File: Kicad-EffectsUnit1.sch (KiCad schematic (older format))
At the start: 109 parts, among them J101 In7, J102 Doepfer connector, J103 Vin 7-12v, J104 In6, J105 In3, J106 Out10, J107 Out11, J108 Out12, J109 Out13, J110 Power Conn, SW101 Dist 10, SW102 Crush A3, SW103 Rotary_Encoder_Switch, SW104 Dist 12, U101 TL072, U102 TL072

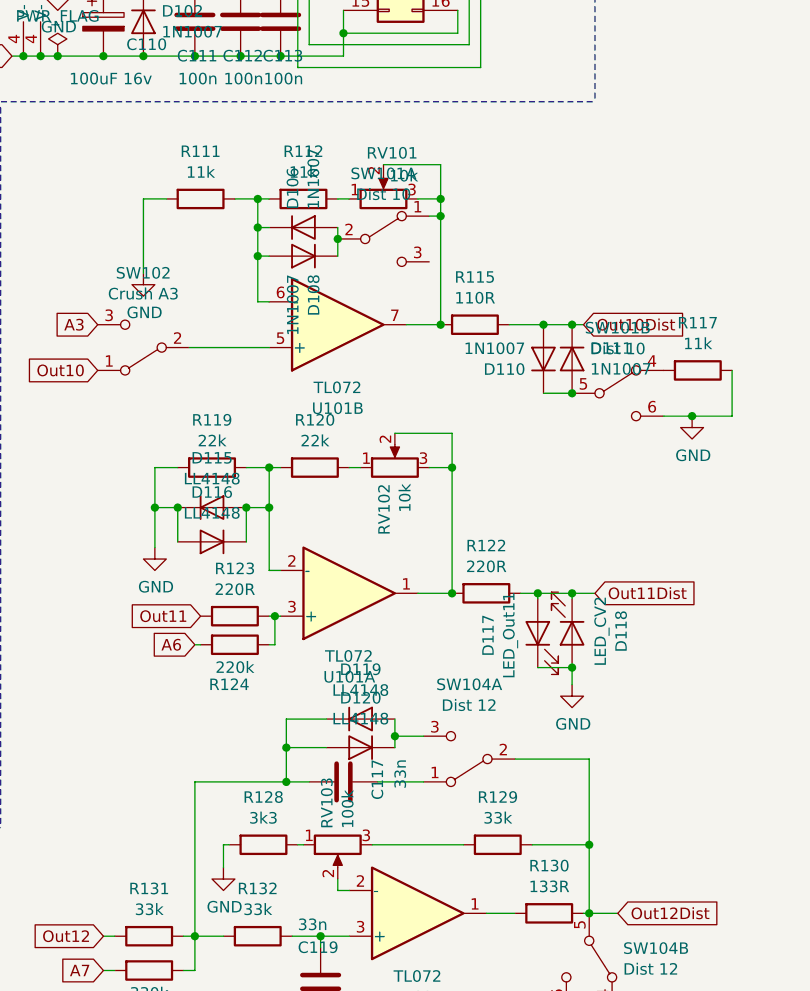
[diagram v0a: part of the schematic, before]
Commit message: Footprints
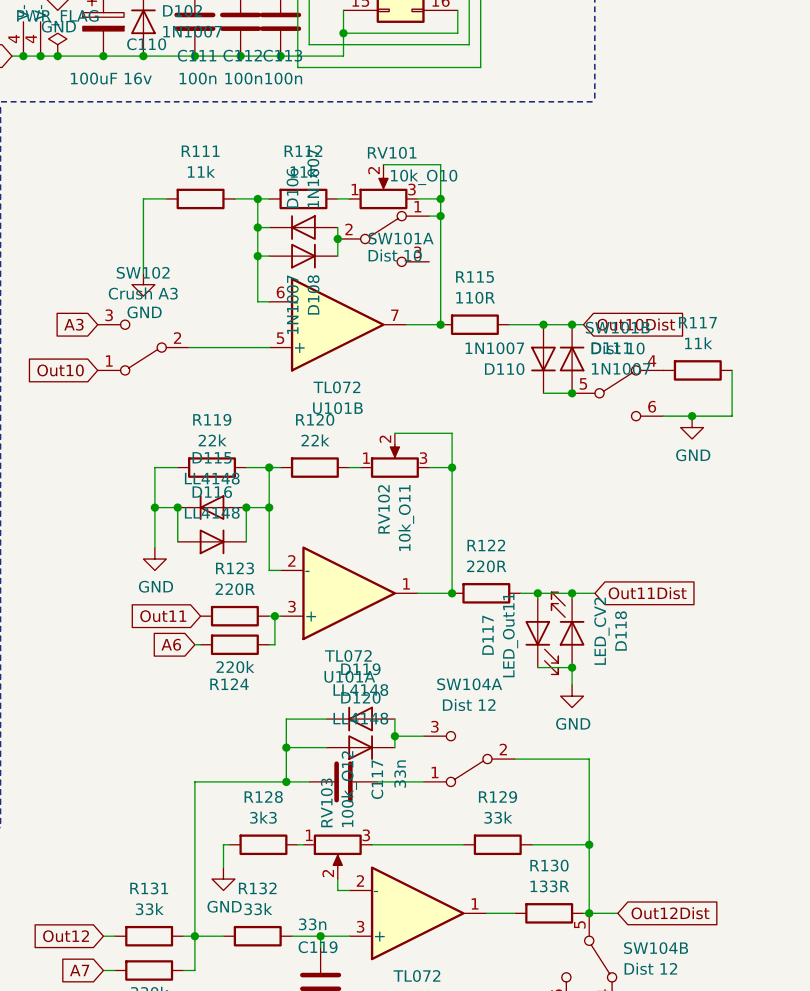
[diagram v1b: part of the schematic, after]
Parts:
- RV101: value 10k -> 10k_O10; footprint Potentiometer_THT:Potentiometer_Alps_RK09K_Single_Vertical -> Potentiometer_THT:Potentiometer_China_RK09_Single_Vertical_AJ
- RV102: value 10k -> 10k_O11; footprint Potentiometer_THT:Potentiometer_Alps_RK09K_Single_Vertical -> Potentiometer_THT:Potentiometer_China_RK09_Single_Vertical_AJ
- RV103: value 100k -> 100k_O12; footprint Potentiometer_THT:Potentiometer_Alps_RK09K_Single_Vertical -> Potentiometer_THT:Potentiometer_China_RK09_Single_Vertical_AJ
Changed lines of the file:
@@
 P 5375 3400
 F 0 "RV102" H 5305 3446 50  0000 R CNN
-F 1 "10k" H 5305 3355 50  0000 R CNN
-F 2 "Potentiometer_THT:Potentiometer_Alps_RK09K_Single_Vertical" H 5375 3400 50  0001 C CNN
+F 1 "10k_O11" H 5305 3355 50  0000 R CNN
+F 2 "Potentiometer_THT:Potentiometer_China_RK09_Single_Vertical_AJ" H 5375 3400 50  0001 C CNN
 F 3 "~" H 5375 3400 50  0001 C CNN
 	1    5375 3400
@@
 P 5325 2225
 F 0 "RV101" V 5525 2300 50  0000 R CNN
-F 1 "10k" V 5425 2200 50  0000 R CNN
-F 2 "Potentiometer_THT:Potentiometer_Alps_RK09K_Single_Vertical" H 5325 2225 50  0001 C CNN
+F 1 "10k_O10" V 5425 2200 50  0000 R CNN
+F 2 "Potentiometer_THT:Potentiometer_China_RK09_Single_Vertical_AJ" H 5325 2225 50  0001 C CNN
 F 3 "~" H 5325 2225 50  0001 C CNN
 	1    5325 2225
@@
 U 1 1 5D077A76
 P 5325 2400
-F 0 "SW101" H 5325 2685 50  0000 C CNN
-F 1 "Dist 10" H 5325 2594 50  0000 C CNN
+F 0 "SW101" H 5400 2400 50  0000 C CNN
+F 1 "Dist 10" H 5375 2325 50  0000 C CNN
 F 2 "AJ-Dropbox-Kicad:SPDTx2" H 5325 2400 50  0001 C CNN
 F 3 "~" H 5325 2400 50  0001 C CNN
@@
 P 5125 5050
 F 0 "RV103" H 5055 5096 50  0000 R CNN
-F 1 "100k" H 5055 5005 50  0000 R CNN
-F 2 "Potentiometer_THT:Potentiometer_Alps_RK09K_Single_Vertical" H 5125 5050 50  0001 C CNN
+F 1 "100k_O12" H 5055 5005 50  0000 R CNN
+F 2 "Potentiometer_THT:Potentiometer_China_RK09_Single_Vertical_AJ" H 5125 5050 50  0001 C CNN
 F 3 "~" H 5125 5050 50  0001 C CNN
 	1    5125 5050
